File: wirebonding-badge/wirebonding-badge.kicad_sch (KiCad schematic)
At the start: 14 parts, among them SW1 SW_Push, SW2 SW_Push, SW3 SW_Push, SW4 SW_Push, U2 LM2576HVS-3.3

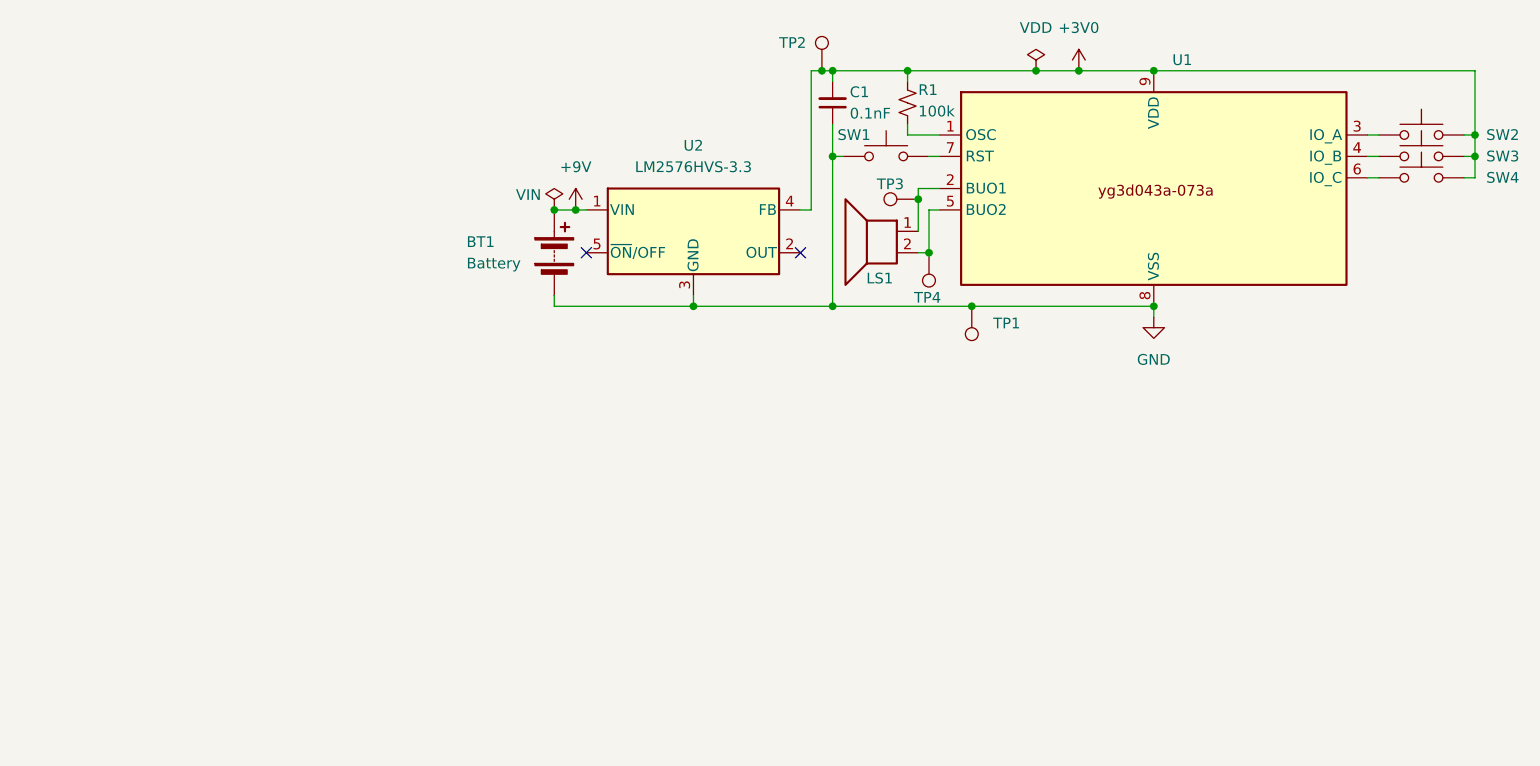
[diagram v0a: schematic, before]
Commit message: Final revision for 5/2025.
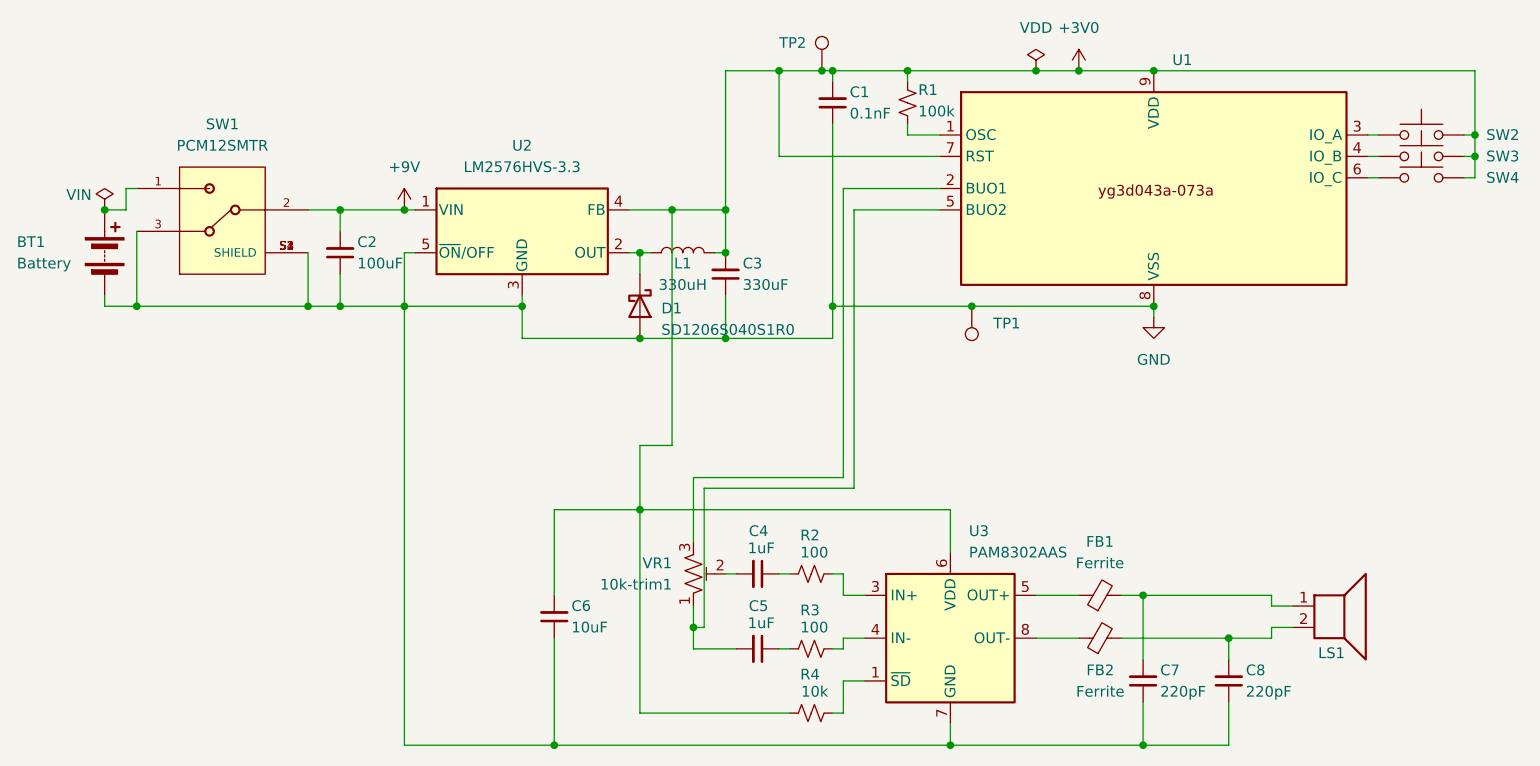
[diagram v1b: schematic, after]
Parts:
- removed SW1: SW_Push, Button_Switch_SMD:SW_Push_1TS009xxxx-xxxx-xxxx_6x6x5mm, symbol Switch:SW_Push
- removed TP3, TP4: TestPoint, TestPoint:TestPoint_Keystone_5019_Minature, symbol Connector:TestPoint
- added 10k-trim1: VR1, Resistor_SMD:TRIM_TC33X-2-102E, symbol Device:R_Potentiometer_Trim_US
- added C2: 100uF, Capacitor_SMD:C_1206_3216Metric, symbol Device:C_Small
- added C3: 330uF, Capacitor_SMD:C_1206_3216Metric, symbol Device:C_Small
- added C4, C5: 1uF, Capacitor_SMD:C_1206_3216Metric, symbol Device:C_Small
- added C6: 10uF, Capacitor_SMD:C_1206_3216Metric, symbol Device:C_Small
- added C7, C8: 220pF, Capacitor_SMD:C_1206_3216Metric, symbol Device:C_Small
- added D1: SD1206S040S1R0, Diode_SMD:D_1206_3216Metric_Pad1.42x1.75mm_HandSolder, symbol Device:D_Schottky
- added FB1, FB2: Ferrite, Inductor_SMD:L_1206_3216Metric_Pad1.22x1.90mm_HandSolder, symbol Device:FerriteBead_Small
- added L1: 330uH, Inductor_SMD:L_1206_3216Metric_Pad1.22x1.90mm_HandSolder, symbol Device:L
- added R2, R3: 100, Resistor_SMD:R_1206_3216Metric, symbol Device:R_Small_US
- added R4: 10k, Resistor_SMD:R_1206_3216Metric, symbol Device:R_Small_US
- added SW1: PCM12SMTR, Library:SW_PCM12SMTR, symbol New_Library:PCM12SMTR
- added U3: PAM8302AAS, Package_SO:MSOP-8_3x3mm_P0.65mm, symbol Amplifier_Audio:PAM8302AAS
- LS1: footprint Buzzer_Beeper:Speaker_CUI_CMR-1206S-67 -> Buzzer_Beeper:same_sky_speaker_mix
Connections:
- net +3V0: now also U1.7 (RST), C3.2, C6.2, L1.2, R4.1, U3.6 (VDD)
- net +9V: now also C2.2, SW1.2; no longer BT1.1 (+)
- net GND: now also U2.5 (~{ON}/OFF), C2.1, C3.1, C6.1, C7.1, C8.1, D1.2 (A), SW1.3, SW1.S1 (SHIELD), SW1.S2 (SHIELD), SW1.S3 (SHIELD), SW1.S4 (SHIELD), U3.7 (GND)
- net at U1.2 (BUO1): now also 10k-trim1.3; no longer LS1.1
- net at U1.5 (BUO2): now also 10k-trim1.1, C5.2; no longer LS1.2
- net at U2.2 (OUT): now also D1.1 (K), L1.1
- new net: BT1.1 (+), SW1.1
- new net: R4.2, U3.1 (~{SD})
- new net: R2.2, U3.3 (IN+)
- new net: R3.2, U3.4 (IN-)
- new net: FB1.1, U3.5 (OUT+)
- new net: FB2.1, U3.8 (OUT-)
- new net: C4.1, R2.1
- new net: 10k-trim1.2, C4.2
- new net: C8.2, FB2.2, LS1.2
- new net: C5.1, R3.1
- new net: C7.2, FB1.2, LS1.1
- no-connect marks 2 -> 0
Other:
- moved on the sheet: BT1, LS1, U2
